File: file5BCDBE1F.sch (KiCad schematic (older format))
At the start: 20 parts, among them J3 Jack-DC, Q3 Q_PMOS_DGS, U3 AP2210N-3.3TRG1, U7 TPS630701

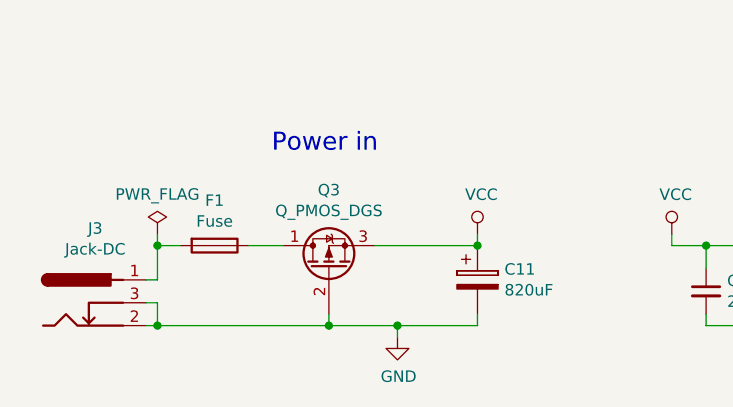
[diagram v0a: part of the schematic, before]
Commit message: Version 4
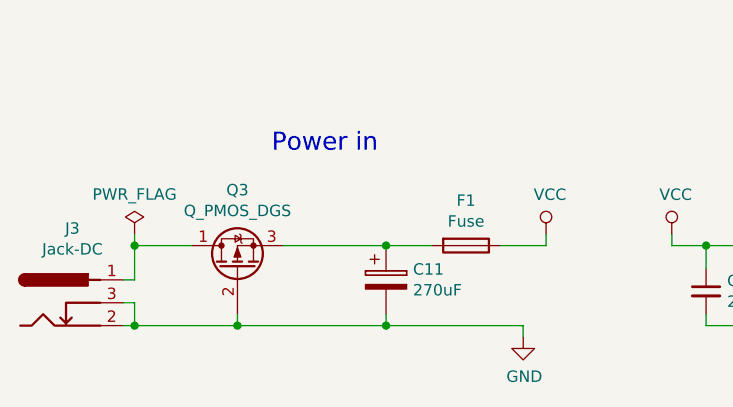
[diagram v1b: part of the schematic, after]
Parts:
- C11: value 820uF -> 270uF; footprint Capacitors_THT:CP_Radial_D10.0mm_P5.00mm -> Capacitors_THT:CP_Radial_D8.0mm_P3.50mm
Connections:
- net VCC: now also F1.1; no longer C11.1, Q3.3 (S)
- net at J3.1: now also Q3.1 (D); no longer F1.2
- new net: C11.1, F1.2, Q3.3 (S)
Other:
- moved on the sheet: C11, F1, J3, Q3
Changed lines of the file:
@@
 EESchema Schematic File Version 4
 LIBS:pi-hat-cache
-EELAYER 26 0
+EELAYER 29 0
 EELAYER END
 $Descr A4 11693 8268
@@
 L pi-hat-rescue:Connector_Specialized_Jack-DC-pi-hat-cache-pi-hat-rescue J?
 U 1 1 5BCDC42E
-P 850 2150
+P 750 2150
 AR Path="/5BCDC42E" Ref="J?"  Part="1"
 AR Path="/5BCDBE20/5BCDC42E" Ref="J3"  Part="1"
-F 0 "J3" H 928 2475 50  0000 C CNN
-F 1 "Jack-DC" H 928 2384 50  0000 C CNN
-F 2 "Connectors:BARREL_JACK" H 900 2110 50  0001 C CNN
-F 3 "~" H 900 2110 50  0001 C CNN
-F 4 "CP-002A-ND" H 850 2150 50  0001 C CNN "Digikey"
-F 5 "https://www.digikey.com/product-detail/en/cui-inc/PJ-002A/CP-002A-ND/96962" H -200 -400 50  0001 C CNN "Link"
-F 6 "PJ-002A" H -200 -400 50  0001 C CNN "MPN"
-F 7 "DC-005" H -200 -400 50  0001 C CNN "OPL"
-	1    850  2150
+F 0 "J3" H 828 2475 50  0000 C CNN
+F 1 "Jack-DC" H 828 2384 50  0000 C CNN
+F 2 "Connectors:BARREL_JACK" H 800 2110 50  0001 C CNN
+F 3 "~" H 800 2110 50  0001 C CNN
+F 4 "CP-002A-ND" H 750 2150 50  0001 C CNN "Digikey"
+F 5 "https://www.digikey.com/product-detail/en/cui-inc/PJ-002A/CP-002A-ND/96962" H -300 -400 50  0001 C CNN "Link"
+F 6 "PJ-002A" H -300 -400 50  0001 C CNN "MPN"
+F 7 "DC-005" H -300 -400 50  0001 C CNN "OPL"
+	1    750  2150
 	1    0    0    -1
 $EndComp
@@
 L pi-hat-rescue:CP-Device-pi-hat-rescue C?
 U 1 1 5BCDC46F
-P 2600 2050
+P 2200 2050
 AR Path="/5BCDC46F" Ref="C?"  Part="1"
 AR Path="/5BCDBE20/5BCDC46F" Ref="C11"  Part="1"
-F 0 "C11" H 2718 2096 50  0000 L CNN
-F 1 "820uF" H 2718 2005 50  0000 L CNN
-F 2 "Capacitors_THT:CP_Radial_D10.0mm_P5.00mm" H 2638 1900 50  0001 C CNN
-F 3 "~" H 2600 2050 50  0001 C CNN
-F 4 "1189-2915-ND" H 2600 2050 50  0001 C CNN "Digikey"
-F 5 "https://www.digikey.com/product-detail/en/rubycon/25ZLH820MEFC10X20/1189-2915-ND/3563817" H 850 -400 50  0001 C CNN "Link"
-F 6 "25ZLH820MEFC10X20" H 850 -400 50  0001 C CNN "MPN"
-	1    2600 2050
+F 0 "C11" H 2318 2096 50  0000 L CNN
+F 1 "270uF" H 2318 2005 50  0000 L CNN
+F 2 "Capacitors_THT:CP_Radial_D8.0mm_P3.50mm" H 2238 1900 50  0001 C CNN
+F 3 "~" H 2200 2050 50  0001 C CNN
+F 4 "1189-2915-ND" H 2200 2050 50  0001 C CNN "Digikey"
+F 5 "https://www.digikey.com/product-detail/en/rubycon/25ZLH820MEFC10X20/1189-2915-ND/3563817" H 450 -400 50  0001 C CNN "Link"
+F 6 "25ZLH820MEFC10X20" H 450 -400 50  0001 C CNN "MPN"
+	1    2200 2050
 	1    0    0    -1
 $EndComp
@@
 L power:VCC #PWR?
 U 1 1 5BCDC47F
-P 2600 1850
+P 2900 1850
 AR Path="/5BCDC47F" Ref="#PWR?"  Part="1"
 AR Path="/5BCDBE20/5BCDC47F" Ref="#PWR020"  Part="1"
-F 0 "#PWR020" H 2600 1700 50  0001 C CNN
-F 1 "VCC" H 2617 2023 50  0000 C CNN
-F 2 "" H 2600 1850 50  0001 C CNN
-F 3 "" H 2600 1850 50  0001 C CNN
-	1    2600 1850
-	1    0    0    -1
-$EndComp
-Wire Wire Line
-	1150 2050 1200 2050
-Wire Wire Line
-	1150 2150 1200 2150
-Wire Wire Line
-	1200 2150 1200 2250
-Wire Wire Line
-	1150 2250 1200 2250
-Connection ~ 1200 2250
+F 0 "#PWR020" H 2900 1700 50  0001 C CNN
+F 1 "VCC" H 2917 2023 50  0000 C CNN
+F 2 "" H 2900 1850 50  0001 C CNN
+F 3 "" H 2900 1850 50  0001 C CNN
+	1    2900 1850
+	1    0    0    -1
+$EndComp
+Wire Wire Line
+	1050 2050 1100 2050
+Wire Wire Line
+	1050 2150 1100 2150
+Wire Wire Line
+	1100 2150 1100 2250
+Wire Wire Line
+	1050 2250 1100 2250
+Connection ~ 1100 2250
 $Comp
 L power:VCC #PWR?
@@
 L Device:Q_PMOS_DGS Q3
 U 1 1 5C89C5A4
-P 1950 2000
-F 0 "Q3" V 2293 2000 50  0000 C CNN
-F 1 "Q_PMOS_DGS" V 2202 2000 50  0000 C CNN
-F 2 "digikey-footprints:IRF9310PbF" H 2150 2100 50  0001 C CNN
-F 3 "~" H 1950 2000 50  0001 C CNN
-F 4 "IRF9310TRPBFCT-ND" H 0   0   50  0001 C CNN "Digikey"
-F 5 "https://www.digikey.com/products/en?keywords=IRF9310TRPBFCT-ND" H 0   0   50  0001 C CNN "Link"
-F 6 "IRF9310TRPBF" H 0   0   50  0001 C CNN "MPN"
-	1    1950 2000
+P 1550 2000
+F 0 "Q3" V 1893 2000 50  0000 C CNN
+F 1 "Q_PMOS_DGS" V 1802 2000 50  0000 C CNN
+F 2 "digikey-footprints:IRF9310PbF" H 1750 2100 50  0001 C CNN
+F 3 "~" H 1550 2000 50  0001 C CNN
+F 4 "IRF9310TRPBFCT-ND" H -400 0   50  0001 C CNN "Digikey"
+F 5 "https://www.digikey.com/products/en?keywords=IRF9310TRPBFCT-ND" H -400 0   50  0001 C CNN "Link"
+F 6 "IRF9310TRPBF" H -400 0   50  0001 C CNN "MPN"
+	1    1550 2000
 	0    -1   -1   0
 $EndComp
@@
 L Device:Fuse F1
 U 1 1 5C8B932A
-P 1450 1900
-F 0 "F1" V 1253 1900 50  0000 C CNN
-F 1 "Fuse" V 1344 1900 50  0000 C CNN
-F 2 "Resistors_SMD:R_0603_HandSoldering" V 1380 1900 50  0001 C CNN
-F 3 "~" H 1450 1900 50  0001 C CNN
-F 4 "P15125CT-ND" H 0   0   50  0001 C CNN "Digikey"
-F 5 "https://www.digikey.com/product-detail/en/panasonic-electronic-components/ERB-RE5R00V/P15125CT-ND/2796832" H 0   0   50  0001 C CNN "Link"
-F 6 "ERB-RE5R00V" H 0   0   50  0001 C CNN "MPN"
-	1    1450 1900
+P 2550 1900
+F 0 "F1" V 2353 1900 50  0000 C CNN
+F 1 "Fuse" V 2444 1900 50  0000 C CNN
+F 2 "Resistors_SMD:R_0603_HandSoldering" V 2480 1900 50  0001 C CNN
+F 3 "~" H 2550 1900 50  0001 C CNN
+F 4 "P15125CT-ND" H 1100 0   50  0001 C CNN "Digikey"
+F 5 "https://www.digikey.com/product-detail/en/panasonic-electronic-components/ERB-RE5R00V/P15125CT-ND/2796832" H 1100 0   50  0001 C CNN "Link"
+F 6 "ERB-RE5R00V" H 1100 0   50  0001 C CNN "MPN"
+	1    2550 1900
 	0    1    1    0
 $EndComp
@@
 	7350 2250 8250 2250
 Wire Wire Line
-	1200 2250 1950 2250
-Wire Wire Line
-	1200 2050 1200 1900
-Wire Wire Line
-	1200 1900 1300 1900
-Wire Wire Line
-	1600 1900 1750 1900
-Wire Wire Line
-	2150 1900 2600 1900
-Wire Wire Line
-	1950 2200 1950 2250
-Connection ~ 1950 2250
-Wire Wire Line
-	1950 2250 2250 2250
-Wire Wire Line
-	2600 2250 2600 2200
-Wire Wire Line
-	2600 1900 2600 1850
-Connection ~ 2600 1900
-Wire Wire Line
 	4300 2300 4300 2250
 Connection ~ 4300 2250
@@
 L power:GND #PWR019
 U 1 1 5C9FE107
-P 2250 2300
-F 0 "#PWR019" H 2250 2050 50  0001 C CNN
-F 1 "GND" H 2255 2127 50  0000 C CNN
-F 2 "" H 2250 2300 50  0001 C CNN
-F 3 "" H 2250 2300 50  0001 C CNN
-	1    2250 2300
-	1    0    0    -1
-$EndComp
-Wire Wire Line
-	2250 2300 2250 2250
-Connection ~ 2250 2250
-Wire Wire Line
-	2250 2250 2600 2250
+P 2800 2300
+F 0 "#PWR019" H 2800 2050 50  0001 C CNN
+F 1 "GND" H 2805 2127 50  0000 C CNN
+F 2 "" H 2800 2300 50  0001 C CNN
+F 3 "" H 2800 2300 50  0001 C CNN
+	1    2800 2300
+	1    0    0    -1
+$EndComp
+Wire Wire Line
+	2800 2300 2800 2250
 Text HLabel 7950 1000 2    50   Input ~ 0
 5V_Enable
@@
 L power:PWR_FLAG #FLG0102
 U 1 1 5CF57122
-P 1200 1850
-F 0 "#FLG0102" H 1200 1925 50  0001 C CNN
-F 1 "PWR_FLAG" H 1200 2024 50  0000 C CNN
-F 2 "" H 1200 1850 50  0001 C CNN
-F 3 "" H 1200 1850 50  0001 C CNN
-	1    1200 1850
-	1    0    0    -1
-$EndComp
-Wire Wire Line
-	1200 1900 1200 1850
-Connection ~ 1200 1900
+P 1100 1850
+F 0 "#FLG0102" H 1100 1925 50  0001 C CNN
+F 1 "PWR_FLAG" H 1100 2024 50  0000 C CNN
+F 2 "" H 1100 1850 50  0001 C CNN
+F 3 "" H 1100 1850 50  0001 C CNN
+	1    1100 1850
+	1    0    0    -1
+$EndComp
 $Comp
 L Device:R R10
@@
 	8250 1450 8250 1800
 Connection ~ 8250 1800
+Wire Wire Line
+	1100 2250 1550 2250
+Wire Wire Line
+	1550 2200 1550 2250
+Connection ~ 1550 2250
+Wire Wire Line
+	2700 1900 2900 1900
+Wire Wire Line
+	2900 1900 2900 1850
+Connection ~ 2200 1900
+Wire Wire Line
+	1550 2250 2200 2250
+Wire Wire Line
+	2200 2200 2200 2250
+Connection ~ 2200 2250
+Wire Wire Line
+	2200 2250 2800 2250
+Wire Wire Line
+	1100 1850 1100 1900
+Wire Wire Line
+	2200 1900 2400 1900
+Wire Wire Line
+	1750 1900 2200 1900
+Wire Wire Line
+	1350 1900 1100 1900
+Connection ~ 1100 1900
+Wire Wire Line
+	1100 1900 1100 2050
 $EndSCHEMATC
